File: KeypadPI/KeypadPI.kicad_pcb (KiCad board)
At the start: 2 copper layers, 100 x 100 mm, 105 parts, among them J1 Conn_01x04, J2 Conn_02x20_Odd_Even, J3 Conn_01x01, J4 Conn_01x01, J5 Conn_01x01, J6 Conn_01x01, J7 Conn_01x04, J8 Conn_01x05, J9 SPEAKER, Q1 2N7000, Q2 2N7000, Q3 2N7000, SW1 SW_Push, SW10 SW_Push, SW11 SW_Push, SW12 SW_Push, SW13 SW_Push, SW14 SW_Push, SW15 SW_Push, SW16 SW_Push, SW2 SW_Push, SW3 SW_Push, SW4 SW_Push, SW5 SW_Push, SW6 SW_Push, SW7 SW_Push, SW8 SW_Push, SW9 SW_Push, U1 74HC595, U2 LM386, U3 LM358, U4 LM358

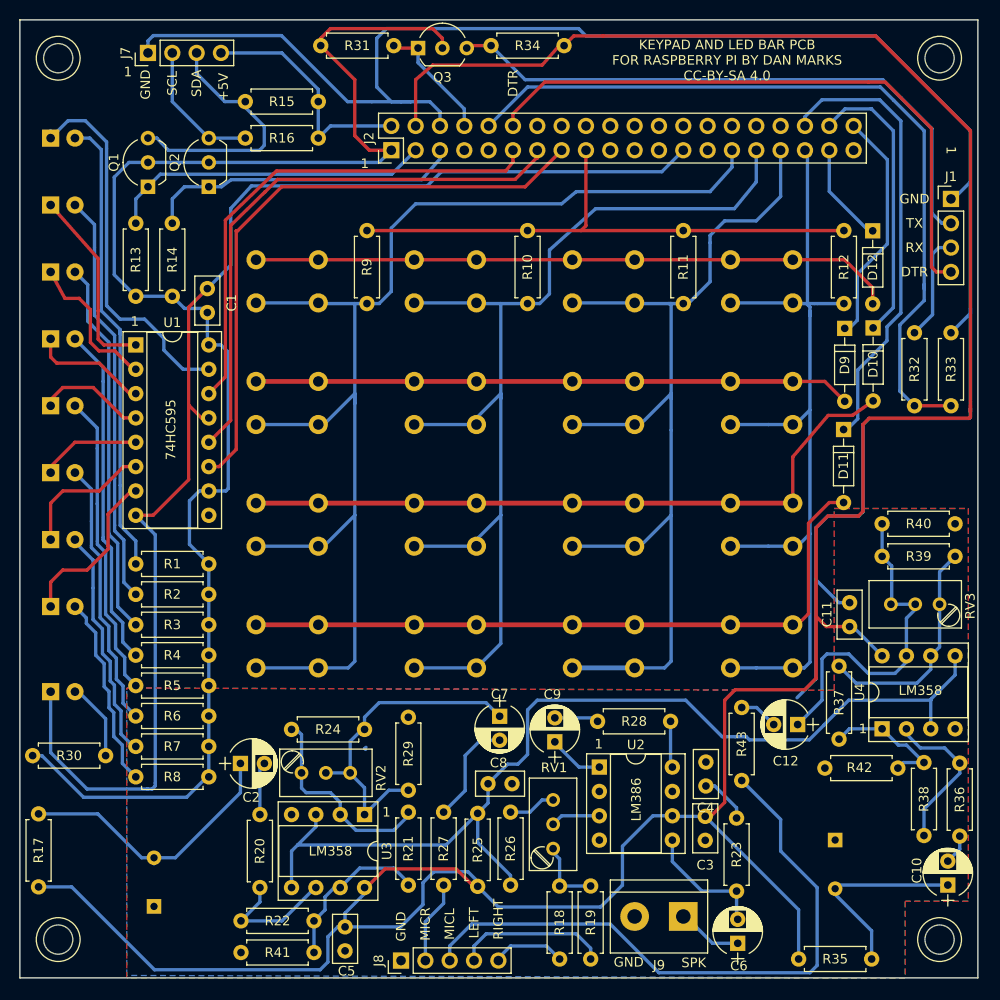
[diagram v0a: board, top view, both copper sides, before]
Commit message: A few fixes
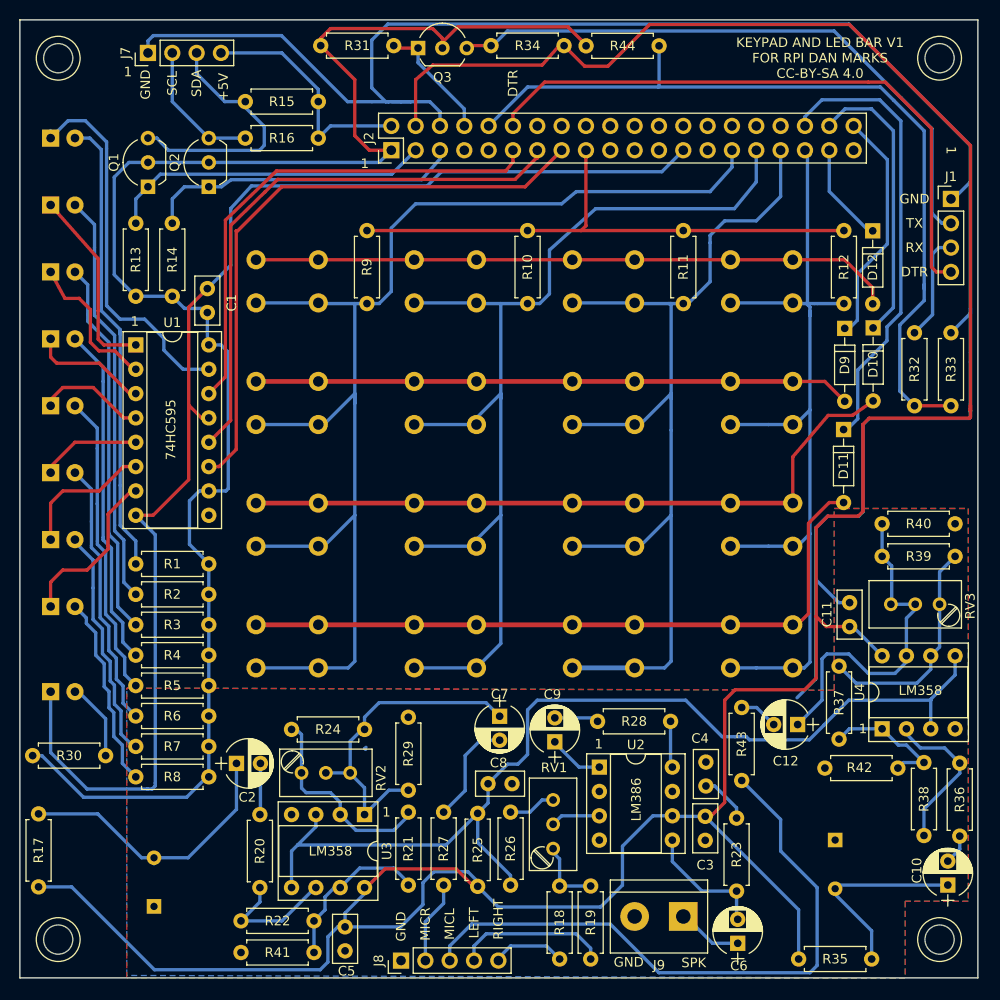
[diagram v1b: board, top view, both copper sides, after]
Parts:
- added R44: NC, Resistors_THT:R_Axial_DIN0207_L6.3mm_D2.5mm_P7.62mm_Horizontal, F.Cu at (92.7, 43.7)
- moved C2 0.41 mm to (48.6, 118.6)
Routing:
- net VCC: track 161.2 -> 178.4 mm
- net /GPIO15UART0RXD: track 83.8 -> 88.1 mm
- net /RPI5V#2: track 300.4 -> 302.8 mm
- net Net-(J1-Pad2): track 64.9 -> 66.2 mm
- net Net-(C2-Pad1): track 29.5 -> 30.1 mm
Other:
- board text added: "KEYPAD AND LED BAR V1 FOR RPI DAN MARKS CC-BY-SA 4.0"
- board text removed: "KEYPAD AND LED BAR PCB FOR RASPBERRY PI BY DAN MARKS CC-BY-SA 4.0"
